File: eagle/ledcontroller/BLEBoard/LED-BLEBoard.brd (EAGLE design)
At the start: 38.4 x 31.7 mm, 19 parts, among them U1 FTSH-105-01-F-DV-ND, U2 RFD22301, U3 TPS61232, U4 V_REG_MIC2920, U5 7AAF-3

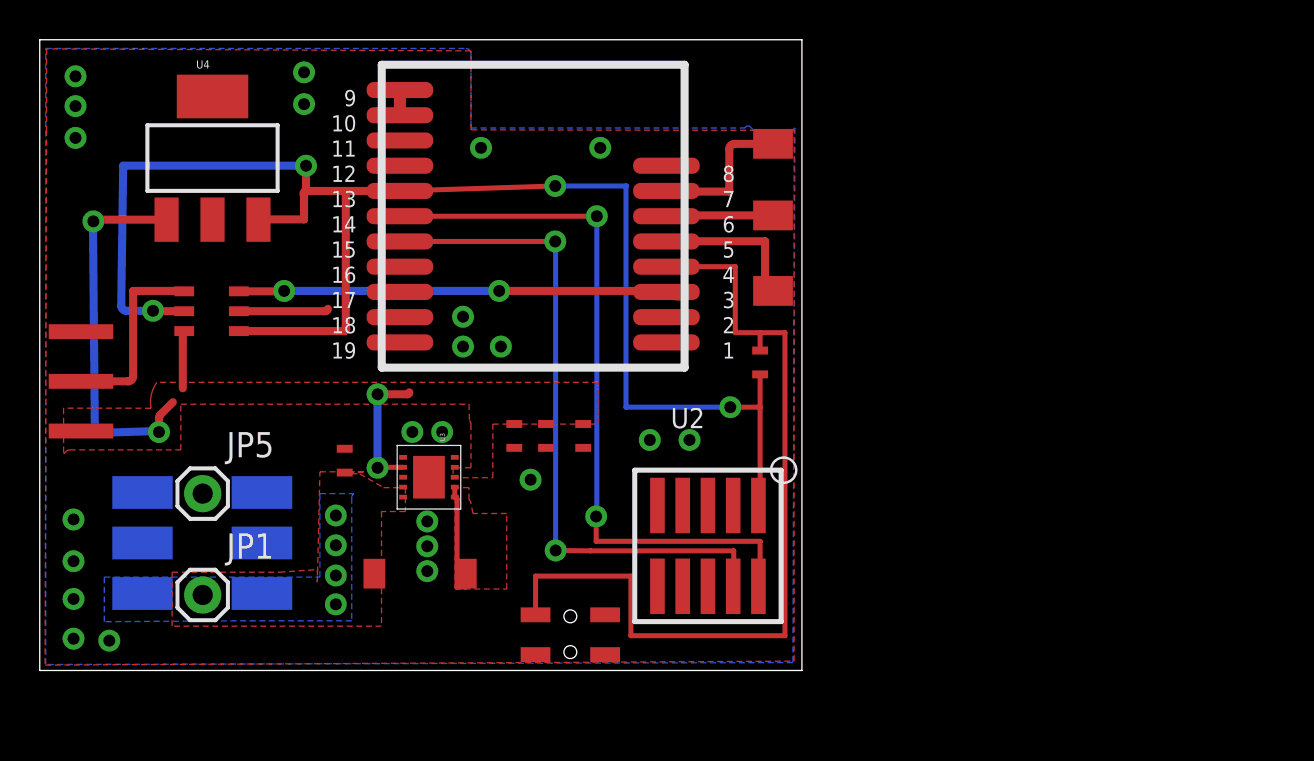
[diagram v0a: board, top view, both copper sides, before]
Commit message: beginning
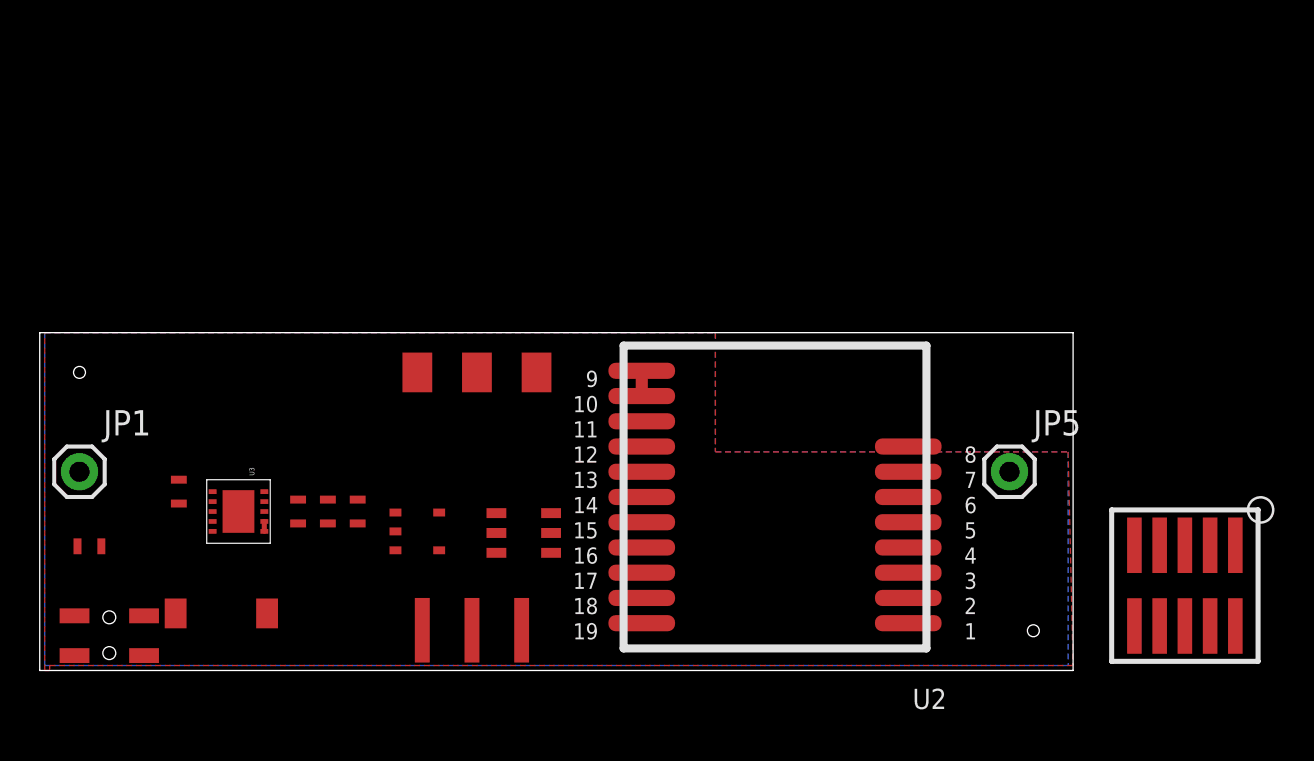
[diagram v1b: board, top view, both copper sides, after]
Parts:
- removed U4: V_REG_MIC2920, SparkFun-PowerIC:SOT223
- U5: value 7AAF-3 -> (none); device bret:70AAJ-3 -> bret:SC-74A-5PIN
- moved JP5 40.6 mm to (48.8, 10.0)
- moved U$4 35.0 mm to (2.50, 6.25), turned to 180 degrees
- moved U1 24.1 mm to (57.6, 4.27)
- moved U$3 23.2 mm to (6.00, 0.50)
- moved JP4 21.3 mm to (19.0, 15.0), turned to 180 degrees
- moved U2 18.6 mm to (37.0, 10.0)
- moved U$1 17.7 mm to (18.0, 0.40), turned to 0 degrees
- moved JP3 16.9 mm to (22.0, 15.0), turned to 180 degrees
- moved U$2 16.2 mm to (23.5, 8.42), turned to 270 degrees
- moved U5 16.1 mm to (19.0, 7.00), flipped to the top, turned to 270 degrees
- moved JP2 12.6 mm to (25.0, 15.0), turned to 180 degrees
- moved C3 12.0 mm to (16.0, 8.00), turned to 270 degrees
- moved C2 11.6 mm to (14.5, 8.00), turned to 270 degrees
- moved C4 11.5 mm to (13.0, 8.00), turned to 270 degrees
- moved L1 10.2 mm to (9.14, 2.87)
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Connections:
- net 3.3V: now also U5.P$5; no longer U4.3
- net GND: now also U5.P$2; no longer U4.2, U5.P$3@1, U5.P$3@3
- net PWR5V: now also U5.P$1, U5.P$3; no longer U4.1
- net VCC: no longer U5.P$1@1, U5.P$1@2
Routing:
- net 3.3V: track 77.8 -> 0.00 mm, vias 4 -> 0
- net N$2: track 42.9 -> 0.00 mm
- net N$3: track 36.9 -> 0.00 mm, vias 2 -> 0
- net N$1: track 34.2 -> 0.00 mm, vias 2 -> 0
- net PWR5V: track 29.7 -> 0.00 mm, vias 4 -> 0
- net GPIO2: track 24.0 -> 0.00 mm, vias 2 -> 0
- net N$10: track 9.60 -> 0.00 mm
- net GPIO4: track 7.72 -> 0.00 mm
- net GPIO6: track 7.63 -> 0.00 mm
- net PWIND: track 6.16 -> 0.50 mm
- net GPIO5: track 5.38 -> 0.00 mm
- net GND: track 5.80 -> 1.27 mm, vias 23 -> 0
- removed copper zone on layer 1, net PWIND
- removed copper zone on layer 1, net PWR5V
- removed copper zone on layer 1, net VCC
- removed copper zone on layer 16, net VCC
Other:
- board size 38.4 x 31.7 mm -> 52 x 17 mm
- board text removed: "2.3-5.5v"
- board text removed: "C1"
- board text removed: "Copyright 2015, Bret Patterson"
- board text removed: "GND"
- board text removed: "GPIO4"
- board text removed: "GPIO5"
- board text removed: "GPIO6"
- board text removed: "LED Controller REV A"
